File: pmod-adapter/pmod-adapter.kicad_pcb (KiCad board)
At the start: 2 copper layers, 15 parts, among them J1 Conn_01x08, J2 Conn_01x02, J3 Conn_02x06_Top_Bottom, U1 FXMA108BQX, U2 MIC5365-3.3YC5-TR

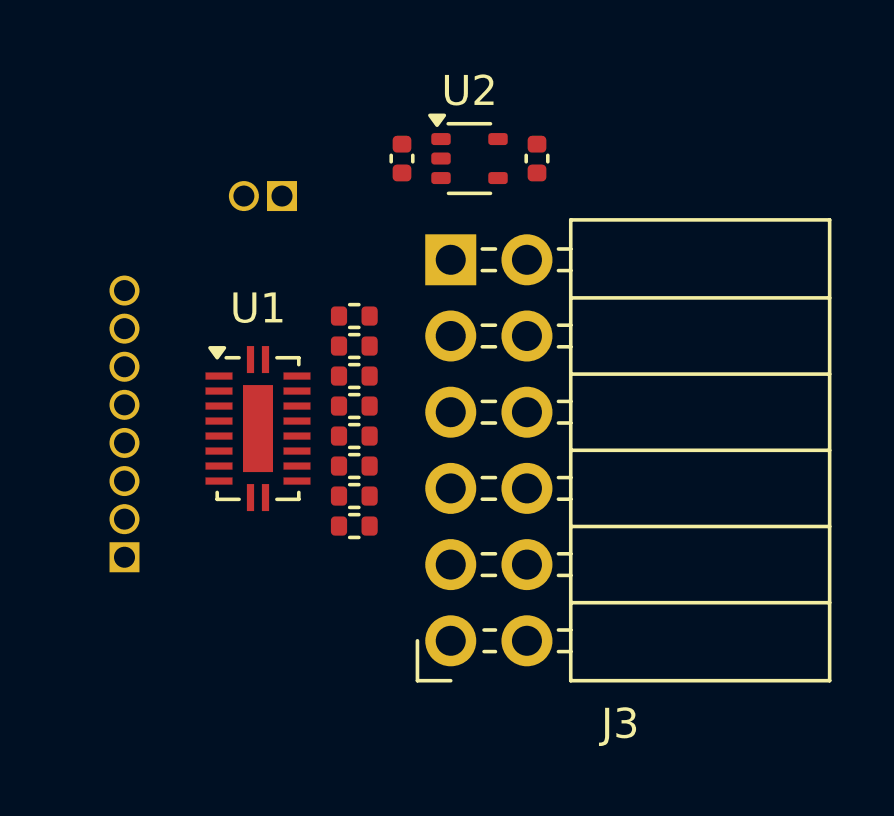
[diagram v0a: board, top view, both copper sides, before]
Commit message: pmod-adapter: Finish board design
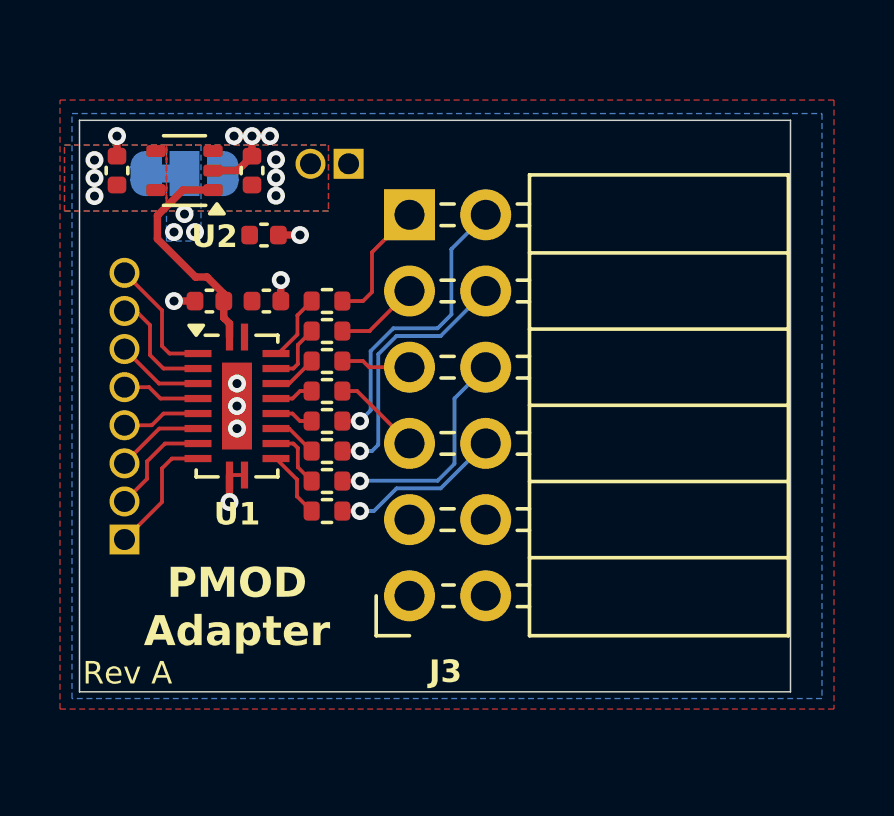
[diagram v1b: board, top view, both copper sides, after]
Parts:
- added C3: 1u, Capacitor_SMD:C_0402_1005Metric, F.Cu at (151.9, 102.8)
- added C4: 100n, Capacitor_SMD:C_0402_1005Metric, F.Cu at (150.1, 105.0)
- added C5: 100n, Capacitor_SMD:C_0402_1005Metric, F.Cu at (152.0, 105.0)
- added JP1: SolderJumper_3_Bridged12, Jumper:SolderJumper-3_P1.3mm_Bridged12_RoundedPad1.0x1.5mm, B.Cu at (149.2, 100.8)
- moved C2 14.0 mm to (147.0, 100.7), turned to 90 degrees
- moved U2 9.51 mm to (149.2, 100.7), turned to 180 degrees
- moved C1 5.02 mm to (151.5, 100.7), turned to 90 degrees
- moved J2 2.47 mm to (154.7, 100.4)
- moved J3 2.03 mm to (156.8, 114.8)
- moved R1 1.04 mm to (154.0, 105.0)
- moved R2 1.04 mm to (154.0, 106.0)
- moved R3 1.04 mm to (154.0, 107.0)
- moved R4 1.04 mm to (154.0, 108.0)
- moved R5 1.04 mm to (154.0, 109.0)
- moved R6 1.04 mm to (154.0, 110.0)
- moved R7 1.04 mm to (154.0, 111.0)
- moved R8 1.04 mm to (154.0, 112.0)
- moved U1 1.03 mm to (151.0, 108.5)
- moved J1 0.59 mm to (147.2, 113.0)
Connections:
- J3 pad 12: +3V3 -> V_{PMOD}
- J3 pad 6: +3V3 -> V_{PMOD}
- U1 pad 11: unconnected-(U1-~{OE}-Pad11) -> GND
- U1 pad 20: +3V3 -> V_{PMOD}
- U1 pad 21: unconnected-(U1-NC-Pad21) -> GND
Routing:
- net /PMOD4: track 0.00 -> 10.1 mm, vias 0 -> 1
- net /PMOD5: track 0.00 -> 8.76 mm, vias 0 -> 1
- net /PMOD6: track 0.00 -> 7.63 mm, vias 0 -> 1
- net GND: track 0.00 -> 7.56 mm, vias 0 -> 11
- net +5V: track 0.00 -> 7.47 mm, vias 0 -> 3
- net /PMOD7: track 0.00 -> 5.71 mm, vias 0 -> 1
- net Net-(J1-Pin_8): track 0.00 -> 4.26 mm
- net Net-(J1-Pin_1): track 0.00 -> 4.22 mm
- net /PMOD0: track 0.00 -> 4.21 mm
- net Net-(J1-Pin_7): track 0.00 -> 3.83 mm
- net Net-(J1-Pin_2): track 0.00 -> 3.59 mm
- net /PMOD3: track 0.00 -> 2.96 mm
- net Net-(J1-Pin_3): track 0.00 -> 2.93 mm
- net Net-(J1-Pin_6): track 0.00 -> 2.93 mm
- net /PMOD1: track 0.00 -> 2.79 mm
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- added copper zone on B.Cu, net +3V3
- added copper zone on F.Cu, net +3V3
- added copper zone on B.Cu, net +5V
- added copper zone on F.Cu, net +5V
- added copper zone on B.Cu, net GND
- added copper zone on B.Cu, net V_{PMOD}
- added copper zone on F.Cu, net V_{PMOD}
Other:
- board outline added: 23.7 x 19.1 mm
- board text added: "3V3"
- board text added: "5V"
- board text added: "PMOD Adapter"
- board text added: "Rev A"
- board text added: "V_{PMOD}"
